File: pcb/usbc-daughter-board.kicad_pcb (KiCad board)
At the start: 2 copper layers, 20.6 x 20.6 mm, 11 parts, among them J1 USBC FS 2.0, J2 JST1x04, U1 USBLC6-2SC6

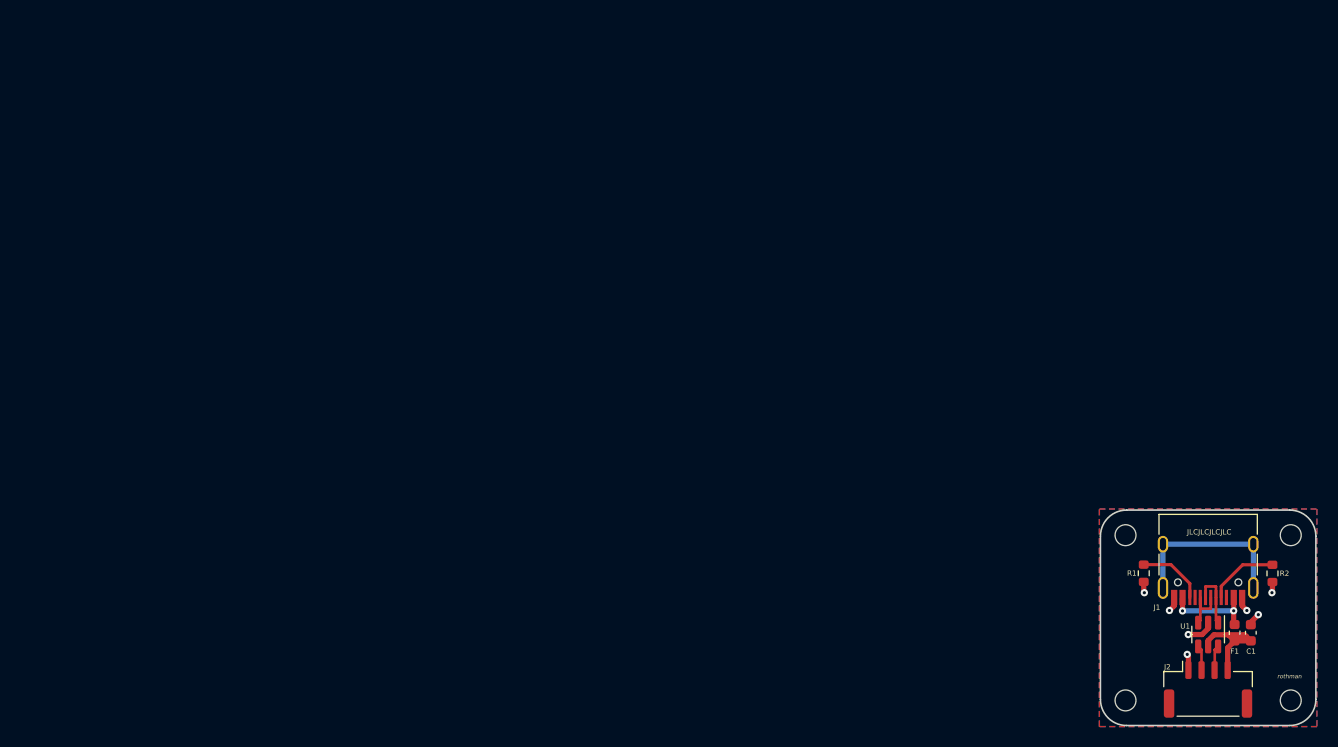
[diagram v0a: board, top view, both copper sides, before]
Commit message: Added gerbers
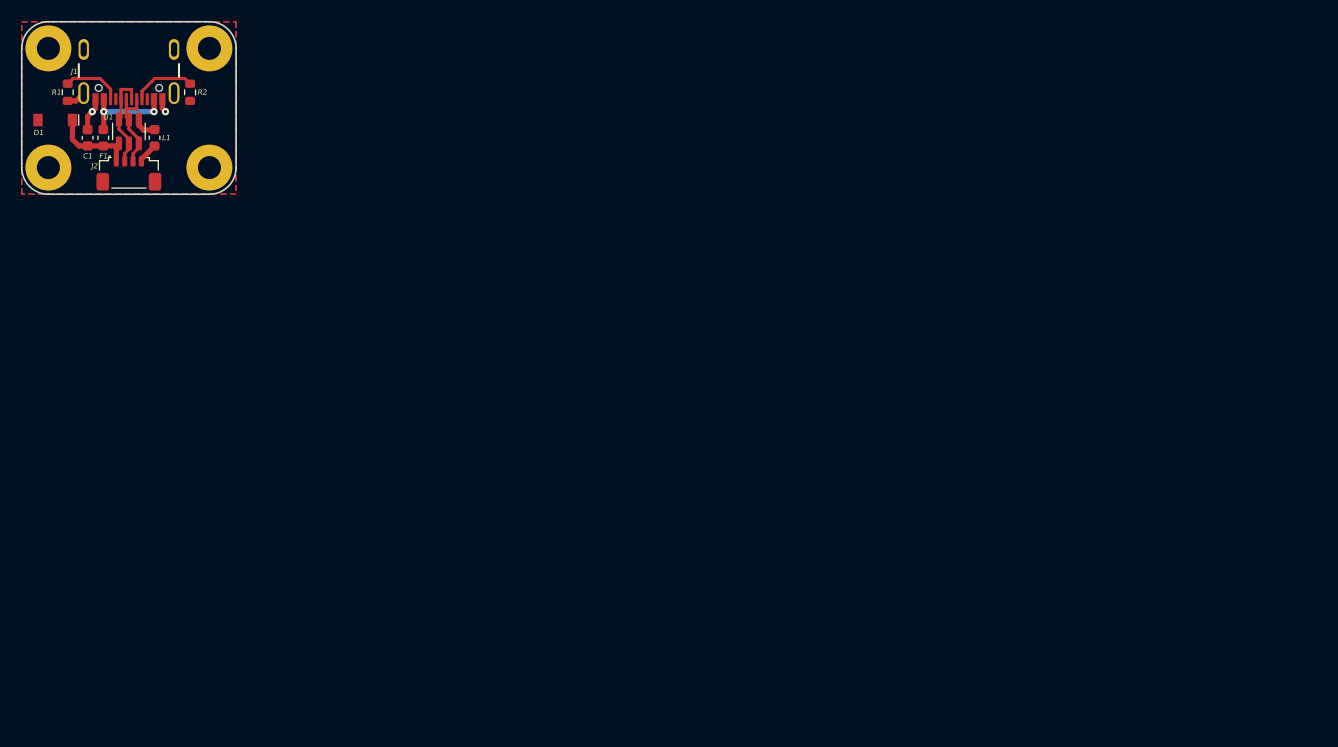
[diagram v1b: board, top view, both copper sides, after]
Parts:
- removed the H2 at (135.4, 63.0)
- removed the H2 at (119.6, 63.0)
- added D1: D_TVS, Diode_SMD:D_SOD-123, F.Cu at (17.2, 23.3)
- added H1: M2, MountingHole:MountingHole_2.2mm_M2_Pad, F.Cu at (16.6, 16.4)
- added H2: M2, MountingHole:MountingHole_2.2mm_M2_Pad, F.Cu at (32.0, 16.4)
- added L1: 60R@100MHz, Inductor_SMD:L_0603_1608Metric, F.Cu at (26.8, 25.0)
- C1: footprint capacitors:C-0603-1608 -> Capacitor_SMD:C_0603_1608Metric
- F1: footprint fuses:Fuse-0603-1608 -> Fuse:Fuse_0603_1608Metric
- H3, H4: value MountingHole -> M2; footprint mechanical:MountingHole-2mm -> MountingHole:MountingHole_2.2mm_M2_Pad
- J1: value USBC FS 2.0 -> USB4105-GF-A; footprint connectors:USB_C_TYPE-C-31-M-12 -> Connector_USB:USB_C_Receptacle_GCT_USB4105-GF-A
- J2: value JST1x04 -> SM04B-SURS-TF; footprint connectors:JST-SM04B-GHS-TB_1x4P -> Connector_JST:JST_SUR_SM04B-SURS-TF_1x04-1MP_P0.80mm_Horizontal
- R1, R2: footprint resistors:R-0603-1608 -> Resistor_SMD:R_0603_1608Metric
- U1: value USBLC6-2SC6 -> TPD4E001; footprint packages:SOT-23-6 -> Package_TO_SOT_SMD:SOT-23-6
- moved C1 120.9 mm to (20.4, 25.0)
- moved F1 118.1 mm to (21.9, 25.0)
- moved H4 115.3 mm to (32.0, 27.9)
- moved H3 114.9 mm to (16.6, 27.9)
- moved J2 114.4 mm to (24.3, 28.4)
- moved J1 114.0 mm to (24.3, 16.6)
- moved U1 113.9 mm to (24.3, 24.4), turned to 90 degrees
- moved R2 113.3 mm to (30.1, 20.6)
- moved R1 112.7 mm to (18.4, 20.6)
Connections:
- C1 pad 2: GND -> GNDPWR
- J1 pad A6: /CON_USB_D+ -> /USB_D+
- J1 pad A7: /CON_USB_D- -> /USB_D-
- J1 pad B6: /CON_USB_D+ -> /USB_D+
- J1 pad B7: /CON_USB_D- -> /USB_D-
- J1 pad S1: unconnected-(J1-PadS1) -> GNDPWR
- J2 pad 1: GND -> VBUS
- J2 pad 2: /JST_USB_D+ -> /USB_D+
- J2 pad 3: /JST_USB_D- -> /USB_D-
- J2 pad 4: VBUS -> GND
- R1 pad 2: GND -> GNDPWR
- R2 pad 2: GND -> GNDPWR
- U1 pad 1: /CON_USB_D- -> VBUS
- U1 pad 2: GND -> /USB_D+
- U1 pad 3: /CON_USB_D+ -> /USB_D-
- U1 pad 4: /JST_USB_D+ -> GNDPWR
- U1 pad 5: VBUS -> /USB_D-
- U1 pad 6: /JST_USB_D- -> /USB_D+
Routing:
- net unconnected-(J1-PadS1): track 17.0 -> 0.00 mm
- net /USB_D+: track 0.00 -> 9.44 mm
- net GNDPWR: track 0.00 -> 8.63 mm, vias 0 -> 2
- net /USB_D-: track 0.00 -> 8.59 mm
- net GND: track 10.5 -> 1.98 mm, vias 7 -> 0
- net /CON_USB_D+: track 5.59 -> 0.00 mm
- net /CON_USB_D-: track 5.58 -> 0.00 mm
- net VBUS: track 11.9 -> 8.47 mm
- net /JST_USB_D-: track 2.40 -> 0.00 mm
- net /JST_USB_D+: track 2.39 -> 0.00 mm
- net /CON_CC2: track 6.49 -> 5.68 mm
- net /CON_CC1: track 6.82 -> 6.06 mm
- added copper zone on B.Cu, net GNDPWR
- added copper zone on F.Cu, net GNDPWR
- removed copper zone on B.Cu, net GND
- removed copper zone on F.Cu, net GND
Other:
- board size 20.6 x 20.6 mm -> 20.5 x 16.5 mm
- rule pad_to_mask_clearance: 0 -> 0.0508
- board text added: "rev1"
- board text removed: "JLCJLCJLCJLC"
